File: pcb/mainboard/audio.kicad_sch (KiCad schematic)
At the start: 29 parts, among them J401 AudioJack3, U201 MIMX8MN6DVTJZAA, U402 FSA2269UMX, U403 WM8978

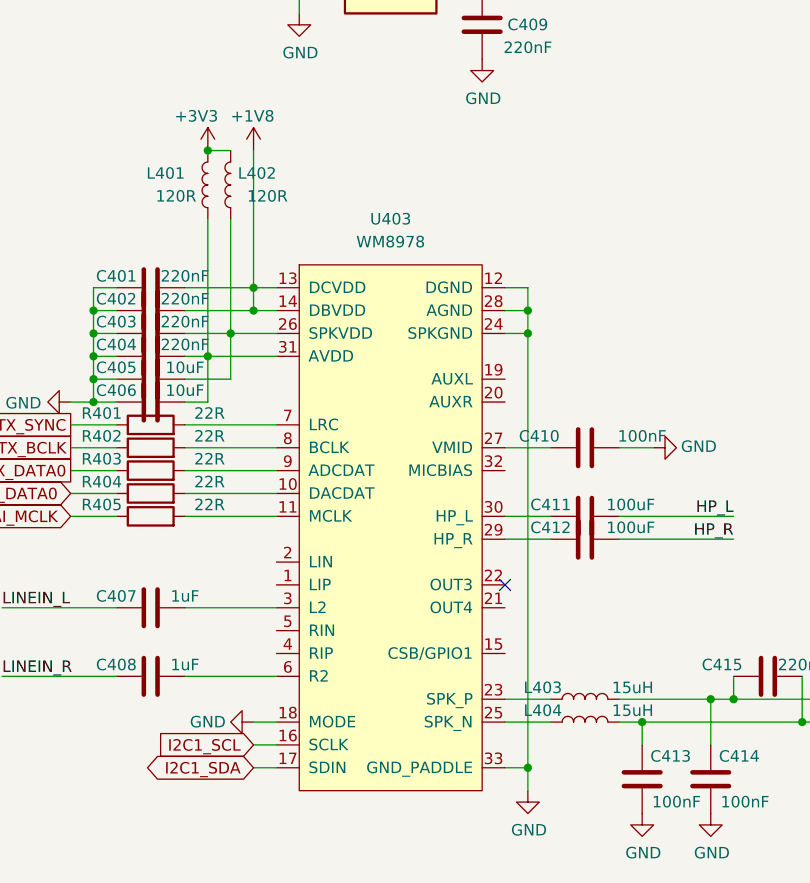
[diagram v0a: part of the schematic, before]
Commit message: Keypad bugfix, pulling in submodules
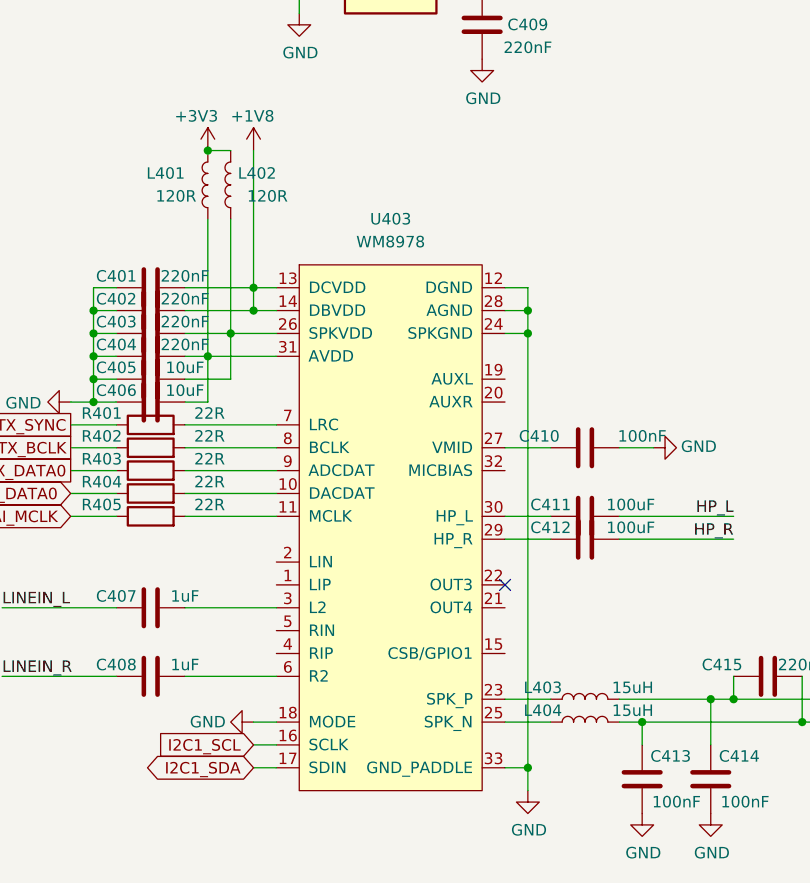
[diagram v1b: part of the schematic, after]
